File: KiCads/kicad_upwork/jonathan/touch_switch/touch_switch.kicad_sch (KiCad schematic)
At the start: 9 parts, among them J1 USB_B, J2 Conn_01x02, J3 Conn_01x02, U1 TTP223-BA6

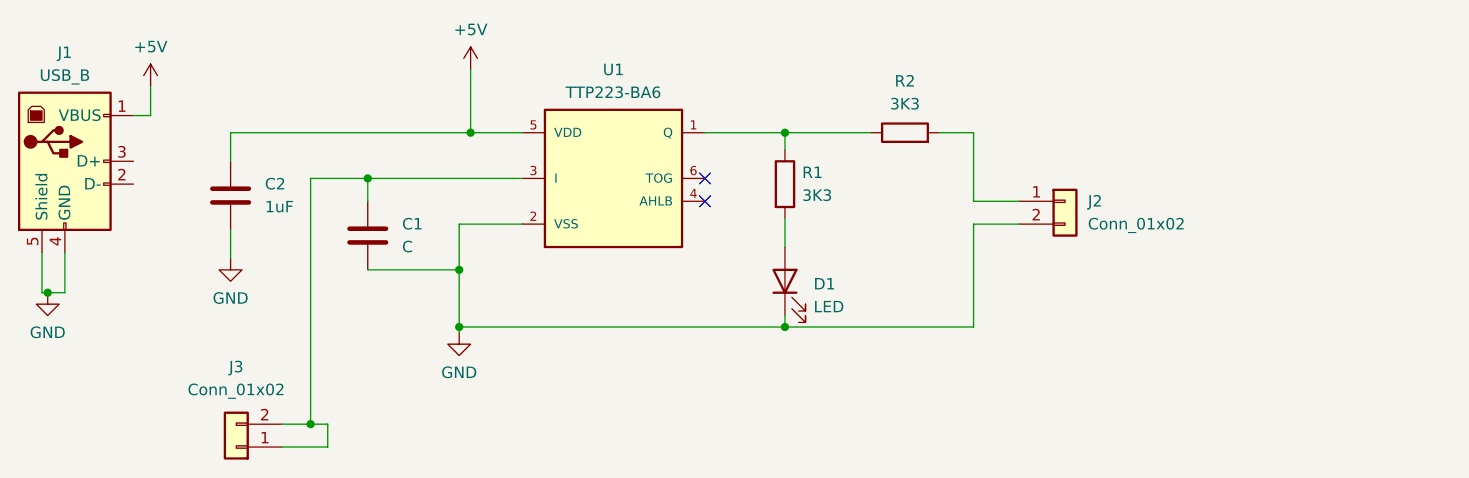
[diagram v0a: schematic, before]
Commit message: 26 Aug 2025 Dorm
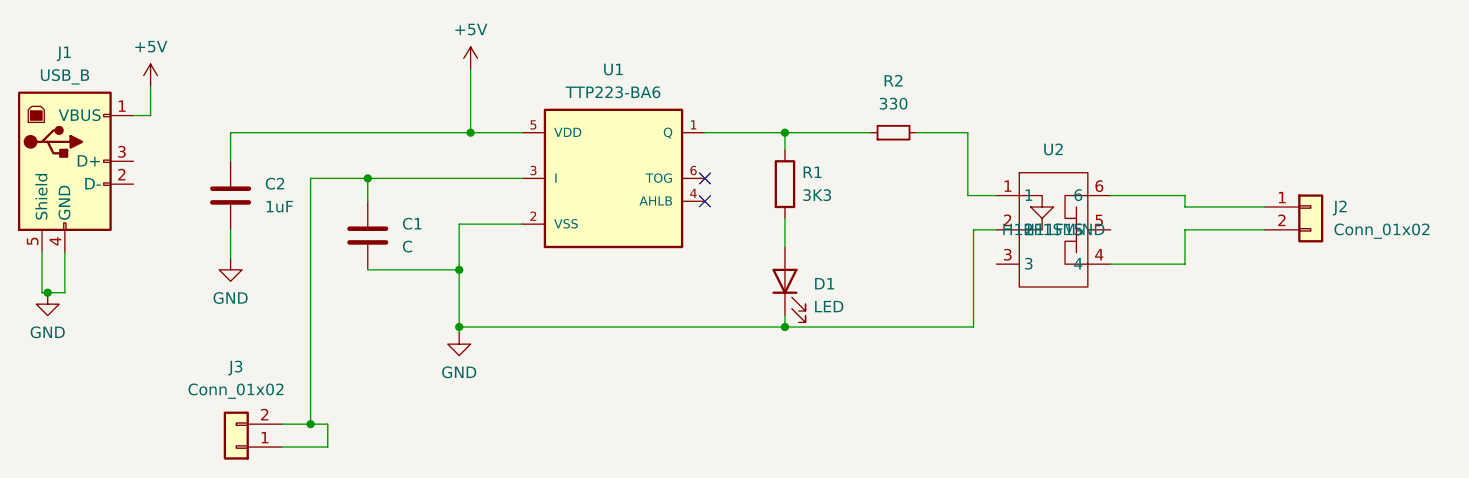
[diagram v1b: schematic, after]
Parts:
- removed R2: 3K3, Resistor_SMD:R_0805_2012Metric, symbol Device:R
- added R2: 330, Resistor_SMD:R_0805_2012Metric, symbol Device:R_Small
- added U2: H11F1S, H11F1SM:OPTOCOUPLER_H11F3SR2M, symbol touch_switch:H11F1S
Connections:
- net GND: now also U2.2; no longer J2.2 (Pin_2)
- net at R1.1, U1.1 (Q): now also R2.1
- net at J2.1 (Pin_1): now also U2.6
- new net: R2.2, U2.1
- new net: J2.2 (Pin_2), U2.4
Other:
- moved on the sheet: J2
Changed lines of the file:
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@@
     (stroke (width 0) (type default))
   )
-  (wire (pts (xy 179.07 85.725) (xy 179.07 97.155))
+  (wire (pts (xy 202.565 83.82) (xy 202.565 82.55))
     (stroke (width 0) (type default))
   )
@@
     (stroke (width 0) (type default))
   )
-  (wire (pts (xy 175.26 75.565) (xy 179.07 75.565))
+  (wire (pts (xy 178.435 75.565) (xy 178.435 82.55))
     (stroke (width 0) (type default))
   )
@@
     (stroke (width 0) (type default))
   )
-  (wire (pts (xy 179.07 75.565) (xy 179.07 83.185))
-    (stroke (width 0) (type default))
-  )
   (wire (pts (xy 158.115 77.47) (xy 158.115 75.565))
     (stroke (width 0) (type default))
   )
+  (wire (pts (xy 202.565 82.55) (xy 194.31 82.55))
+    (stroke (width 0) (type default))
+  )
+  (wire (pts (xy 194.31 90.17) (xy 202.565 90.17))
+    (stroke (width 0) (type default))
+  )
   (wire (pts (xy 123.19 75.565) (xy 128.905 75.565))
     (stroke (width 0) (type default))
@@
     (stroke (width 0) (type default))
   )
+  (wire (pts (xy 181.61 86.36) (xy 179.07 86.36))
+    (stroke (width 0) (type default))
+  )
   (wire (pts (xy 107.315 107.95) (xy 105.41 107.95))
     (stroke (width 0) (type default))
@@
     (stroke (width 0) (type default))
   )
+  (wire (pts (xy 202.565 83.82) (xy 211.455 83.82))
+    (stroke (width 0) (type default))
+  )
   (wire (pts (xy 107.315 110.49) (xy 107.315 107.95))
     (stroke (width 0) (type default))
@@
     (stroke (width 0) (type default))
   )
+  (wire (pts (xy 178.435 82.55) (xy 181.61 82.55))
+    (stroke (width 0) (type default))
+  )
+  (wire (pts (xy 202.565 86.36) (xy 211.455 86.36))
+    (stroke (width 0) (type default))
+  )
   (wire (pts (xy 111.76 80.645) (xy 105.41 80.645))
     (stroke (width 0) (type default))
@@
     (stroke (width 0) (type default))
   )
+  (wire (pts (xy 202.565 90.17) (xy 202.565 86.36))
+    (stroke (width 0) (type default))
+  )
   (wire (pts (xy 128.905 80.645) (xy 111.76 80.645))
     (stroke (width 0) (type default))
@@
     (stroke (width 0) (type default))
   )
-  (wire (pts (xy 184.15 85.725) (xy 179.07 85.725))
+  (wire (pts (xy 172.72 75.565) (xy 178.435 75.565))
     (stroke (width 0) (type default))
   )
@@
     (stroke (width 0) (type default))
   )
-  (wire (pts (xy 179.07 83.185) (xy 184.15 83.185))
+  (wire (pts (xy 179.07 86.36) (xy 179.07 97.155))
     (stroke (width 0) (type default))
   )
@@
     (stroke (width 0) (type default))
   )
-  (symbol (lib_id "Device:R") (at 171.45 75.565 90) (unit 1)
-    (in_bom yes) (on_board yes) (dnp no) (fields_autoplaced)
-    (property "Reference" "R2" (at 171.45 69.85 90)
-      (effects (font (size 1.27 1.27)))
-    )
-    (property "Value" "3K3" (at 171.45 72.39 90)
-      (effects (font (size 1.27 1.27)))
-    )
-    (property "Footprint" "Resistor_SMD:R_0805_2012Metric" (at 171.45 77.343 90)
-      (effects (font (size 1.27 1.27)) hide)
-    )
-    (property "Datasheet" "~" (at 171.45 75.565 0)
-      (effects (font (size 1.27 1.27)) hide)
-    )
-    (property "Supplier Part Number 1" "408-1639-2-ND" (at 171.45 75.565 90)
-      (effects (font (size 1.27 1.27)) hide)
-    )
-    (property "Supplier" "Digikey" (at 171.45 75.565 90)
+  (symbol (lib_id "touch_switch:H11F1S") (at 187.96 86.36 0) (unit 1)
+    (in_bom yes) (on_board yes) (dnp no) (fields_autoplaced)
+    (property "Reference" "U2" (at 187.96 77.47 0)
+      (effects (font (size 1.27 1.27)))
+    )
+    (property "Value" "H11F1S" (at 187.96 86.36 0)
+      (effects (font (size 1.27 1.27)))
+    )
+    (property "Footprint" "H11F1SM:OPTOCOUPLER_H11F3SR2M" (at 189.23 93.98 0)
+      (effects (font (size 1.27 1.27)) hide)
+    )
+    (property "Datasheet" "" (at 187.96 86.36 0)
+      (effects (font (size 1.27 1.27)) hide)
+    )
+    (property "Supplier Part Number 1" "H11F1SM-ND" (at 187.96 86.36 0)
+      (effects (font (size 1.27 1.27)))
+    )
+    (pin "6")
+    (pin "4")
+    (pin "1")
+    (pin "3")
+    (pin "5")
+    (pin "2")
+    (instances
+      (project "touch_switch"
+        (path "/b1a6736c-e9e5-4252-8a05-d0fbb303d9c0"
+          (reference "U2") (unit 1)
+        )
+      )
+    )
+  )
+  (symbol (lib_id "power:GND") (at 121.92 97.79 0) (unit 1)
+    (in_bom yes) (on_board yes) (dnp no) (fields_autoplaced)
+    (property "Reference" "#PWR02" (at 121.92 104.14 0)
+      (effects (font (size 1.27 1.27)) hide)
+    )
+    (property "Value" "GND" (at 121.92 102.235 0)
+      (effects (font (size 1.27 1.27)))
+    )
+    (property "Footprint" "" (at 121.92 97.79 0)
+      (effects (font (size 1.27 1.27)) hide)
+    )
+    (property "Datasheet" "" (at 121.92 97.79 0)
+      (effects (font (size 1.27 1.27)) hide)
+    )
+    (pin "1")
+    (instances
+      (project "touch_switch"
+        (path "/b1a6736c-e9e5-4252-8a05-d0fbb303d9c0"
+          (reference "#PWR02") (unit 1)
+        )
+      )
+    )
+  )
+  (symbol (lib_id "power:GND") (at 76.2 93.345 0) (unit 1)
+    (in_bom yes) (on_board yes) (dnp no) (fields_autoplaced)
+    (property "Reference" "#PWR03" (at 76.2 99.695 0)
+      (effects (font (size 1.27 1.27)) hide)
+    )
+    (property "Value" "GND" (at 76.2 97.79 0)
+      (effects (font (size 1.27 1.27)))
+    )
+    (property "Footprint" "" (at 76.2 93.345 0)
+      (effects (font (size 1.27 1.27)) hide)
+    )
+    (property "Datasheet" "" (at 76.2 93.345 0)
+      (effects (font (size 1.27 1.27)) hide)
+    )
+    (pin "1")
+    (instances
+      (project "touch_switch"
+        (path "/b1a6736c-e9e5-4252-8a05-d0fbb303d9c0"
+          (reference "#PWR03") (unit 1)
+        )
+      )
+    )
+  )
+  (symbol (lib_id "Device:R_Small") (at 170.18 75.565 90) (unit 1)
+    (in_bom yes) (on_board yes) (dnp no) (fields_autoplaced)
+    (property "Reference" "R2" (at 170.18 69.85 90)
+      (effects (font (size 1.27 1.27)))
+    )
+    (property "Value" "330" (at 170.18 72.39 90)
+      (effects (font (size 1.27 1.27)))
+    )
+    (property "Footprint" "Resistor_SMD:R_0805_2012Metric" (at 170.18 75.565 0)
+      (effects (font (size 1.27 1.27)) hide)
+    )
+    (property "Datasheet" "~" (at 170.18 75.565 0)
+      (effects (font (size 1.27 1.27)) hide)
+    )
+    (property "Supplier Part Number 1" "CR0805-JW-331ELFTR-ND" (at 170.18 75.565 90)
       (effects (font (size 1.27 1.27)) hide)
     )
@@
         (path "/b1a6736c-e9e5-4252-8a05-d0fbb303d9c0"
           (reference "R2") (unit 1)
-        )
-      )
-    )
-  )
-  (symbol (lib_id "power:GND") (at 121.92 97.79 0) (unit 1)
-    (in_bom yes) (on_board yes) (dnp no) (fields_autoplaced)
-    (property "Reference" "#PWR02" (at 121.92 104.14 0)
-      (effects (font (size 1.27 1.27)) hide)
-    )
-    (property "Value" "GND" (at 121.92 102.235 0)
-      (effects (font (size 1.27 1.27)))
-    )
-    (property "Footprint" "" (at 121.92 97.79 0)
-      (effects (font (size 1.27 1.27)) hide)
-    )
-    (property "Datasheet" "" (at 121.92 97.79 0)
-      (effects (font (size 1.27 1.27)) hide)
-    )
-    (pin "1")
-    (instances
-      (project "touch_switch"
-        (path "/b1a6736c-e9e5-4252-8a05-d0fbb303d9c0"
-          (reference "#PWR02") (unit 1)
-        )
-      )
-    )
-  )
-  (symbol (lib_id "power:GND") (at 76.2 93.345 0) (unit 1)
-    (in_bom yes) (on_board yes) (dnp no) (fields_autoplaced)
-    (property "Reference" "#PWR03" (at 76.2 99.695 0)
-      (effects (font (size 1.27 1.27)) hide)
-    )
-    (property "Value" "GND" (at 76.2 97.79 0)
-      (effects (font (size 1.27 1.27)))
-    )
-    (property "Footprint" "" (at 76.2 93.345 0)
-      (effects (font (size 1.27 1.27)) hide)
-    )
-    (property "Datasheet" "" (at 76.2 93.345 0)
-      (effects (font (size 1.27 1.27)) hide)
-    )
-    (pin "1")
-    (instances
-      (project "touch_switch"
-        (path "/b1a6736c-e9e5-4252-8a05-d0fbb303d9c0"
-          (reference "#PWR03") (unit 1)
         )
       )
@@
     )
   )
-  (symbol (lib_id "Connector_Generic:Conn_01x02") (at 189.23 83.185 0) (unit 1)
-    (in_bom yes) (on_board yes) (dnp no) (fields_autoplaced)
-    (property "Reference" "J2" (at 191.77 83.185 0)
-      (effects (font (size 1.27 1.27)) (justify left))
-    )
-    (property "Value" "Conn_01x02" (at 191.77 85.725 0)
-      (effects (font (size 1.27 1.27)) (justify left))
-    )
-    (property "Footprint" "TerminalBlock:TerminalBlock_bornier-2_P5.08mm" (at 189.23 83.185 0)
-      (effects (font (size 1.27 1.27)) hide)
-    )
-    (property "Datasheet" "~" (at 189.23 83.185 0)
-      (effects (font (size 1.27 1.27)) hide)
-    )
-    (property "Supplier Part Number 1" "TB006-508-02BE" (at 189.23 83.185 0)
-      (effects (font (size 1.27 1.27)) hide)
-    )
-    (property "Supplier" "Digikey" (at 189.23 83.185 0)
-      (effects (font (size 1.27 1.27)) hide)
-    )
+  (symbol (lib_id "Connector_Generic:Conn_01x02") (at 216.535 83.82 0) (unit 1)
+    (in_bom yes) (on_board yes) (dnp no) (fields_autoplaced)
+    (property "Reference" "J2" (at 219.075 83.82 0)
+      (effects (font (size 1.27 1.27)) (justify left))
+    )
+    (property "Value" "Conn_01x02" (at 219.075 86.36 0)
+      (effects (font (size 1.27 1.27)) (justify left))
+    )
+    (property "Footprint" "TerminalBlock:TerminalBlock_bornier-2_P5.08mm" (at 216.535 83.82 0)
+      (effects (font (size 1.27 1.27)) hide)
+    )
+    (property "Datasheet" "~" (at 216.535 83.82 0)
+      (effects (font (size 1.27 1.27)) hide)
+    )
+    (property "Supplier Part Number 1" "TB006-508-02BE" (at 216.535 83.82 0)
+      (effects (font (size 1.27 1.27)) hide)
+    )
+    (property "Supplier" "Digikey" (at 216.535 83.82 0)
+      (effects (font (size 1.27 1.27)) hide)
+    )
